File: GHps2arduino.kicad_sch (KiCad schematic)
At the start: 20 parts, among them SW1 Green, SW2 Red, SW3 Yellow, SW4 Blue, SW5 Orange, SW6 Start, SW7 Select, SW8 Strum_Up, SW9 Strum_Down, U1 Sparkfun_Pro_Micro

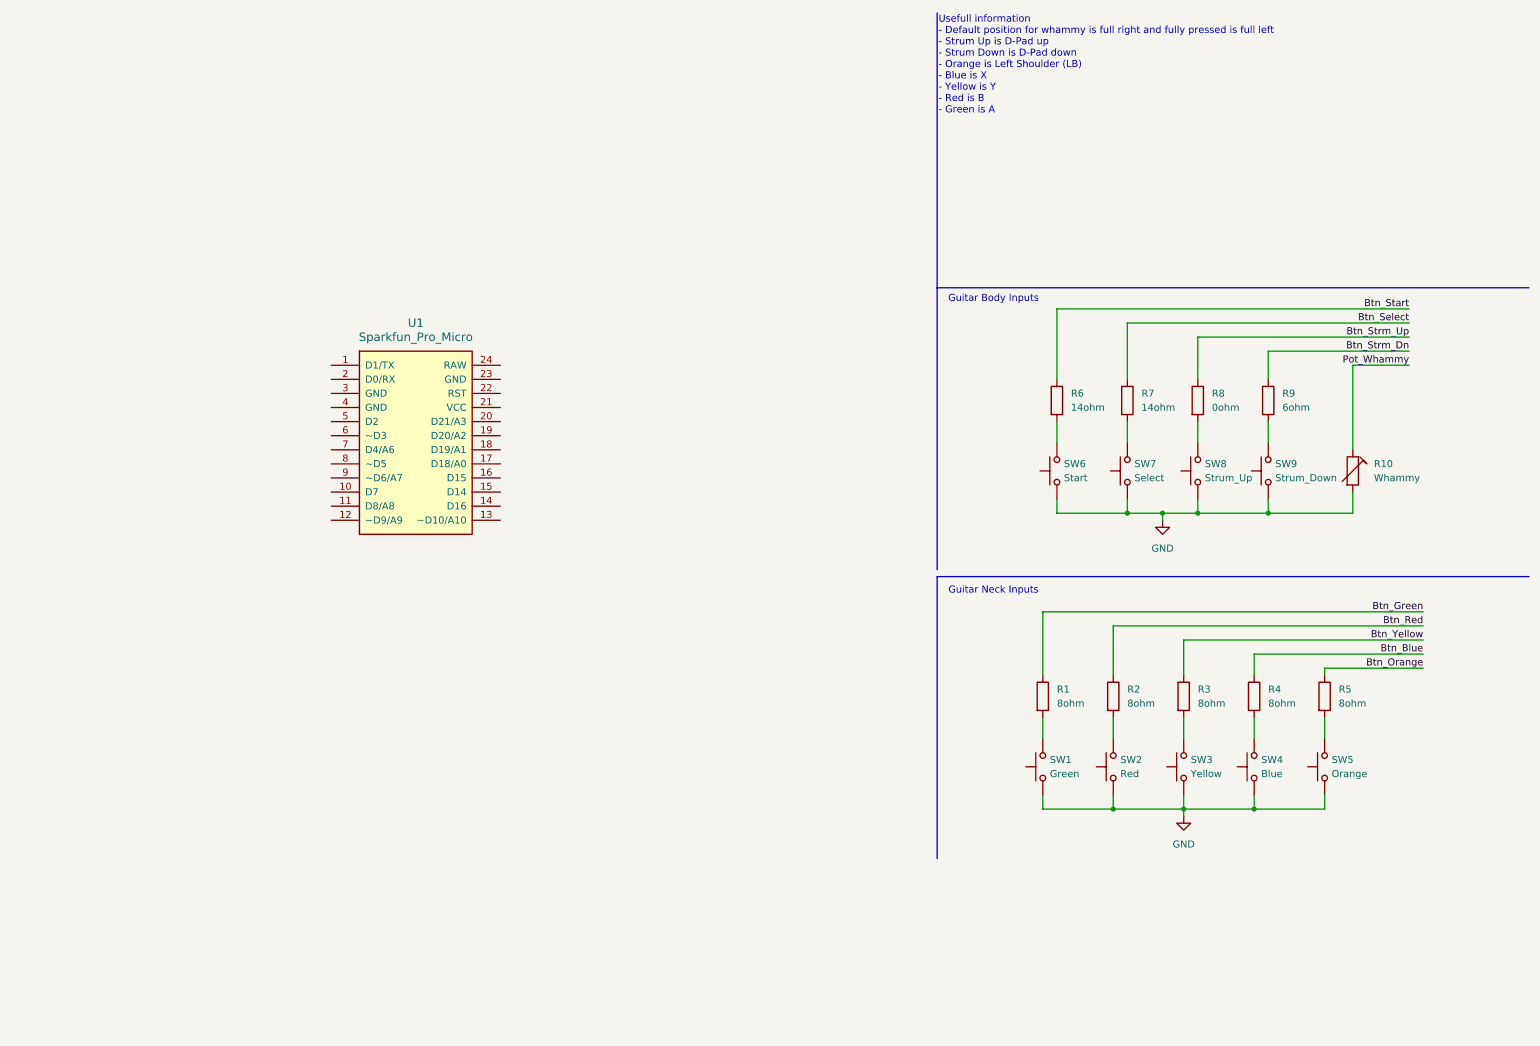
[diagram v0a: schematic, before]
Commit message: Updated With Debounce
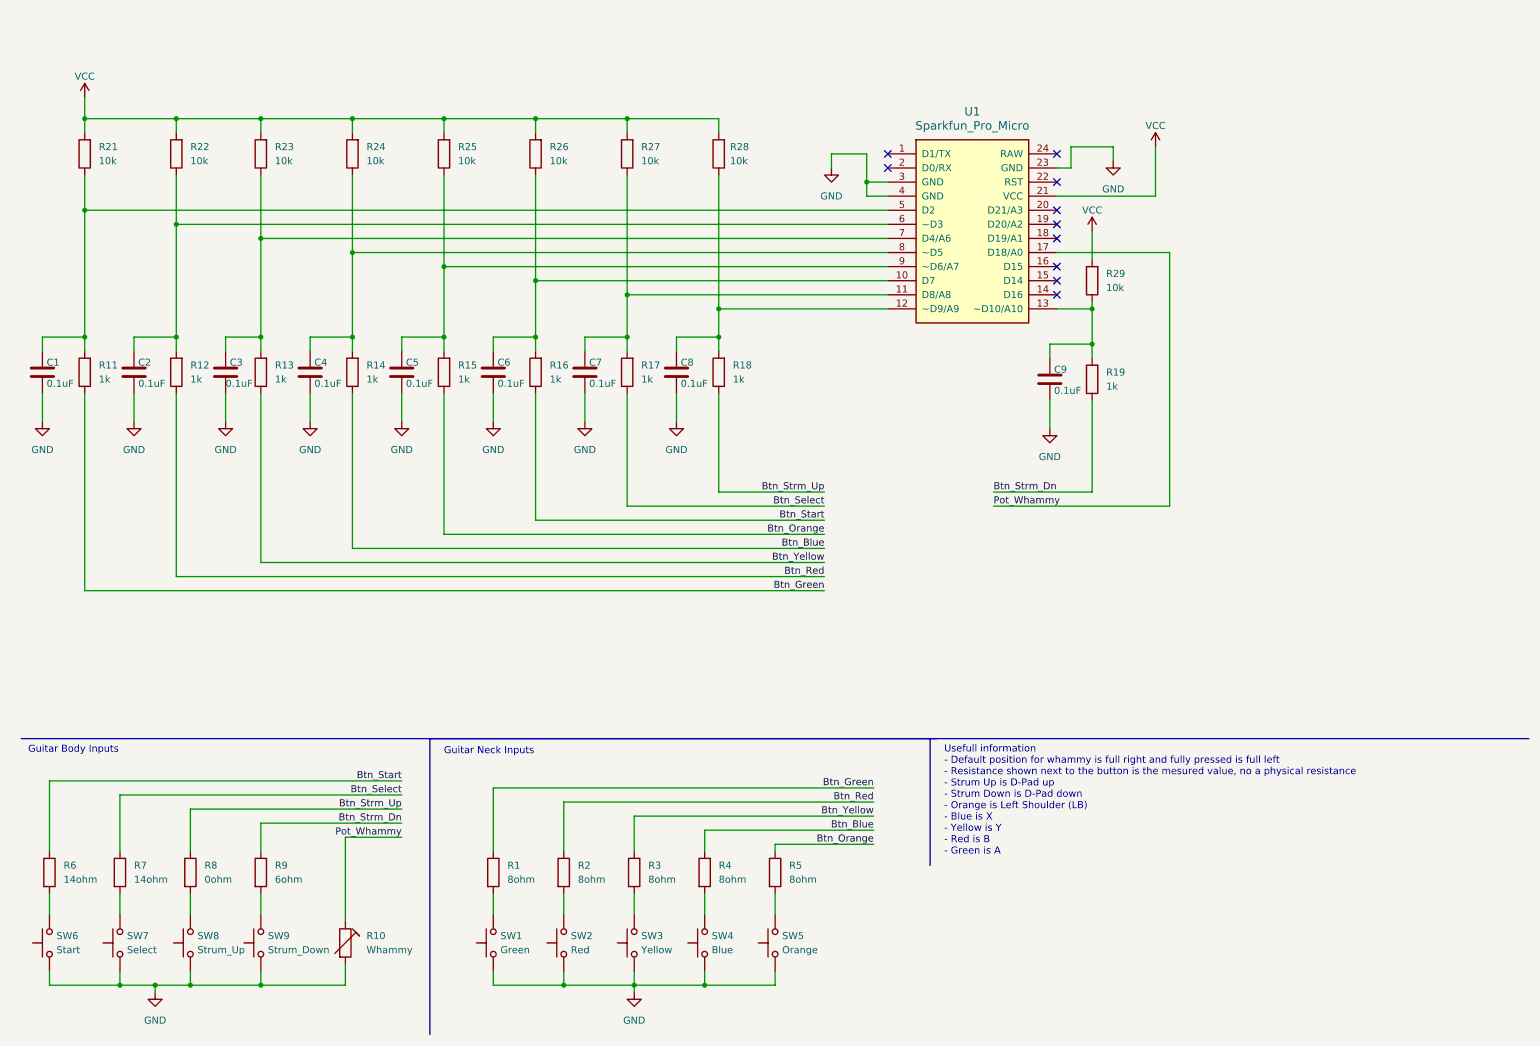
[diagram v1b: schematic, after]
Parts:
- added C1, C2, C3, C4, C5, C6, C7, C8, C9: 0.1uF, symbol Device:C
- added R11, R12, R13, R14, R15, R16, R17, R18, R19: 1k, symbol Device:R
- added R21, R22, R23, R24, R25, R26, R27, R28, R29: 10k, symbol Device:R
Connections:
- net Btn_Blue: now also R14.1
- net Btn_Green: now also R11.1
- net Btn_Orange: now also R15.1
- net Btn_Red: now also R12.1
- net Btn_Select: now also R17.1
- net Btn_Start: now also R16.1
- net Btn_Strm_Dn: now also R19.1
- net Btn_Strm_Up: now also R18.1
- net Btn_Yellow: now also R13.1
- net GND: now also U1.23 (GND), U1.3 (GND), U1.4 (GND), C1.2, C2.2, C3.2, C4.2, C5.2, C6.2, C7.2, C8.2, C9.2
- net Pot_Whammy: now also U1.17 (D18/A0)
- net at U1.10 (D7): now also C6.1, R16.2, R26.1
- net at U1.11 (D8/A8): now also C7.1, R17.2, R27.1
- net at U1.12 (~D9/A9): now also C8.1, R18.2, R28.1
- net at U1.13 (~D10/A10): now also C9.1, R19.2, R29.1
- net VCC: now reaches U1.21 (VCC)
- net VCC: now also R21.2, R22.2, R23.2, R24.2, R25.2, R26.2, R27.2, R28.2, R29.2
- net at U1.5 (D2): now also C1.1, R11.2, R21.1
- net at U1.6 (~D3): now also C2.1, R12.2, R22.1
- net at U1.7 (D4/A6): now also C3.1, R13.2, R23.1
- net at U1.8 (~D5): now also C4.1, R14.2, R24.1
- net at U1.9 (~D6/A7): now also C5.1, R15.2, R25.1
- no-connect marks 0 -> 10
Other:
- note added: "Usefull information - Default position for whammy is full right and fully pressed is full left - Resistance shown next to the button is the mesured value, no a physical resistance - Strum Up is D-Pad up - Strum Down is D-Pad down - Orange is Left Shoulder (LB) - Blue is X - Yellow is Y - Red is B - Green is A"
- note removed: "Usefull information - Default position for whammy is full right and fully pressed is full left - Strum Up is D-Pad up - Strum Down is D-Pad down - Orange is Left Shoulder (LB) - Blue is X - Yellow is Y - Red is B - Green is A"
- title: (none) -> Guitar Hero SG Controller to Arduino Pro Micro Conversion
- moved on the sheet: R1, R10, R2, R3, R4, R5, R6, R7, R8, R9, SW1, SW2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
